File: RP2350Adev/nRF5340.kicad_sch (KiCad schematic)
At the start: 1 part, among them U1 NRF5340-CLAA-R

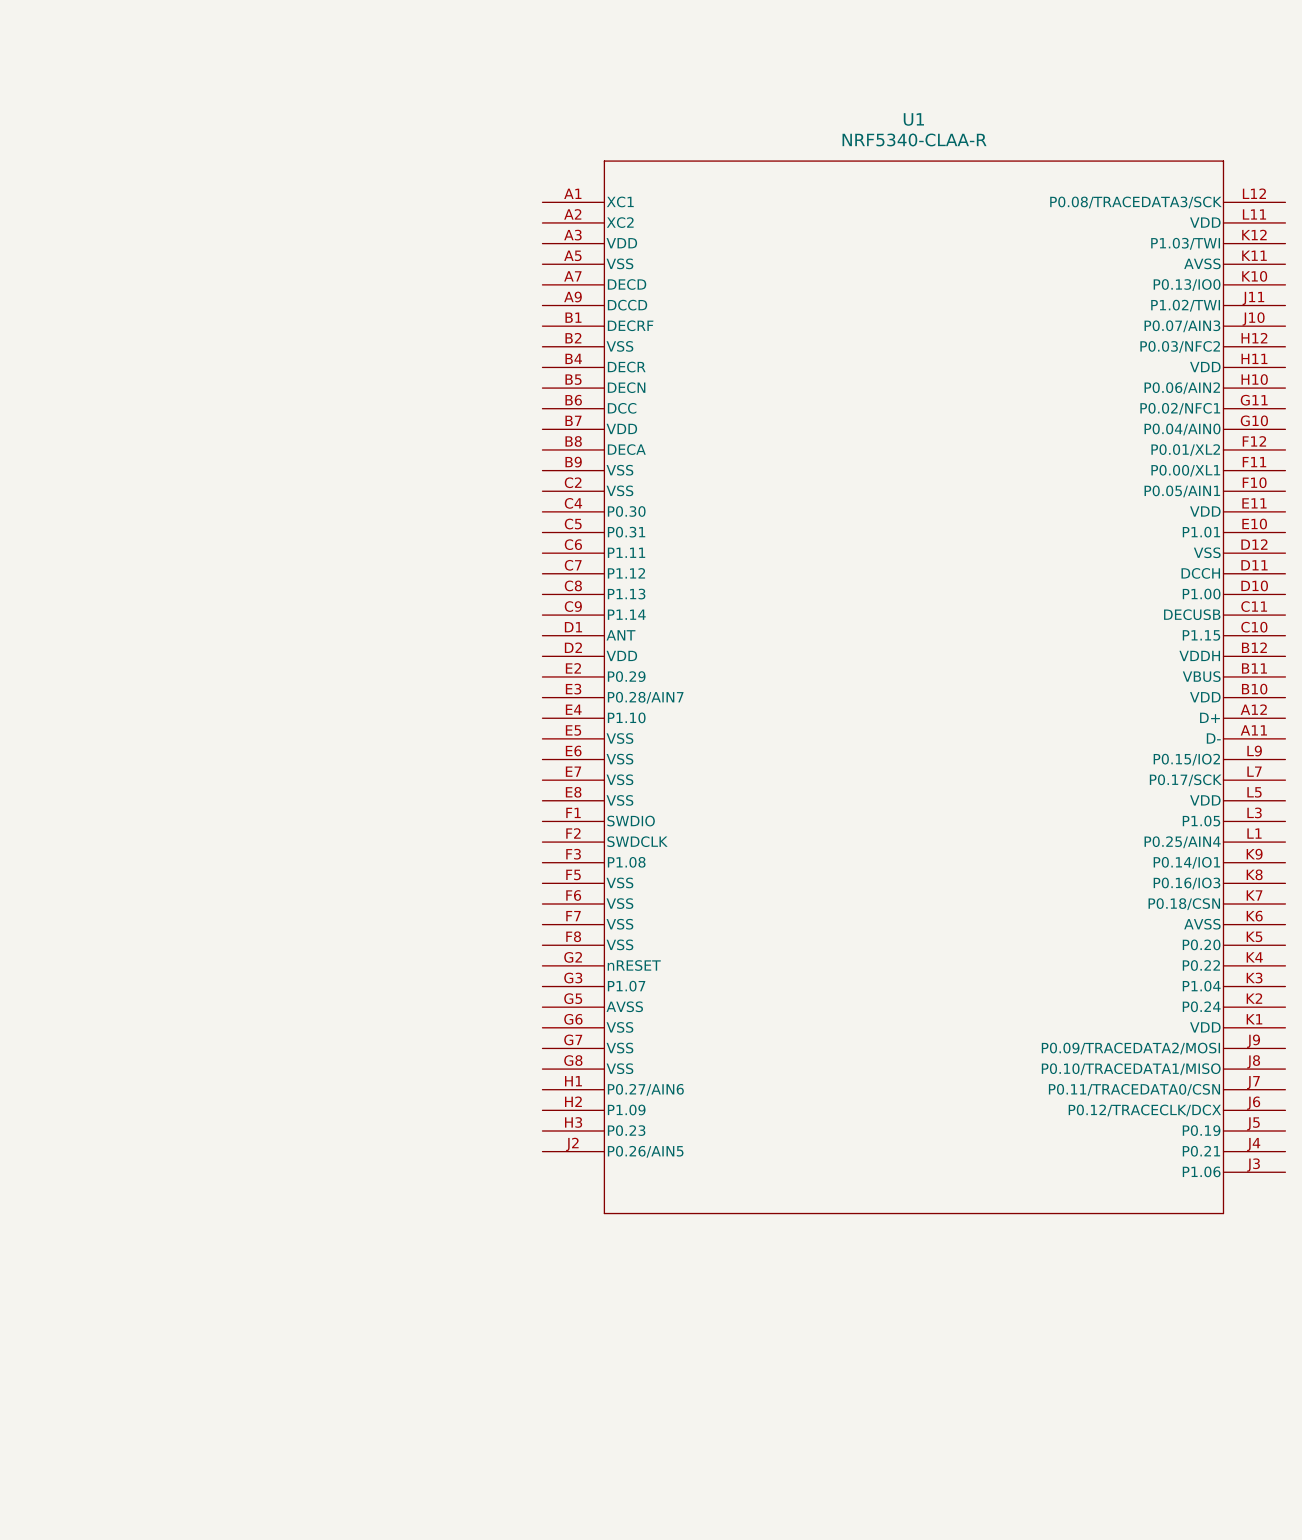
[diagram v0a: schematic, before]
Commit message: Updated nRF5340 work
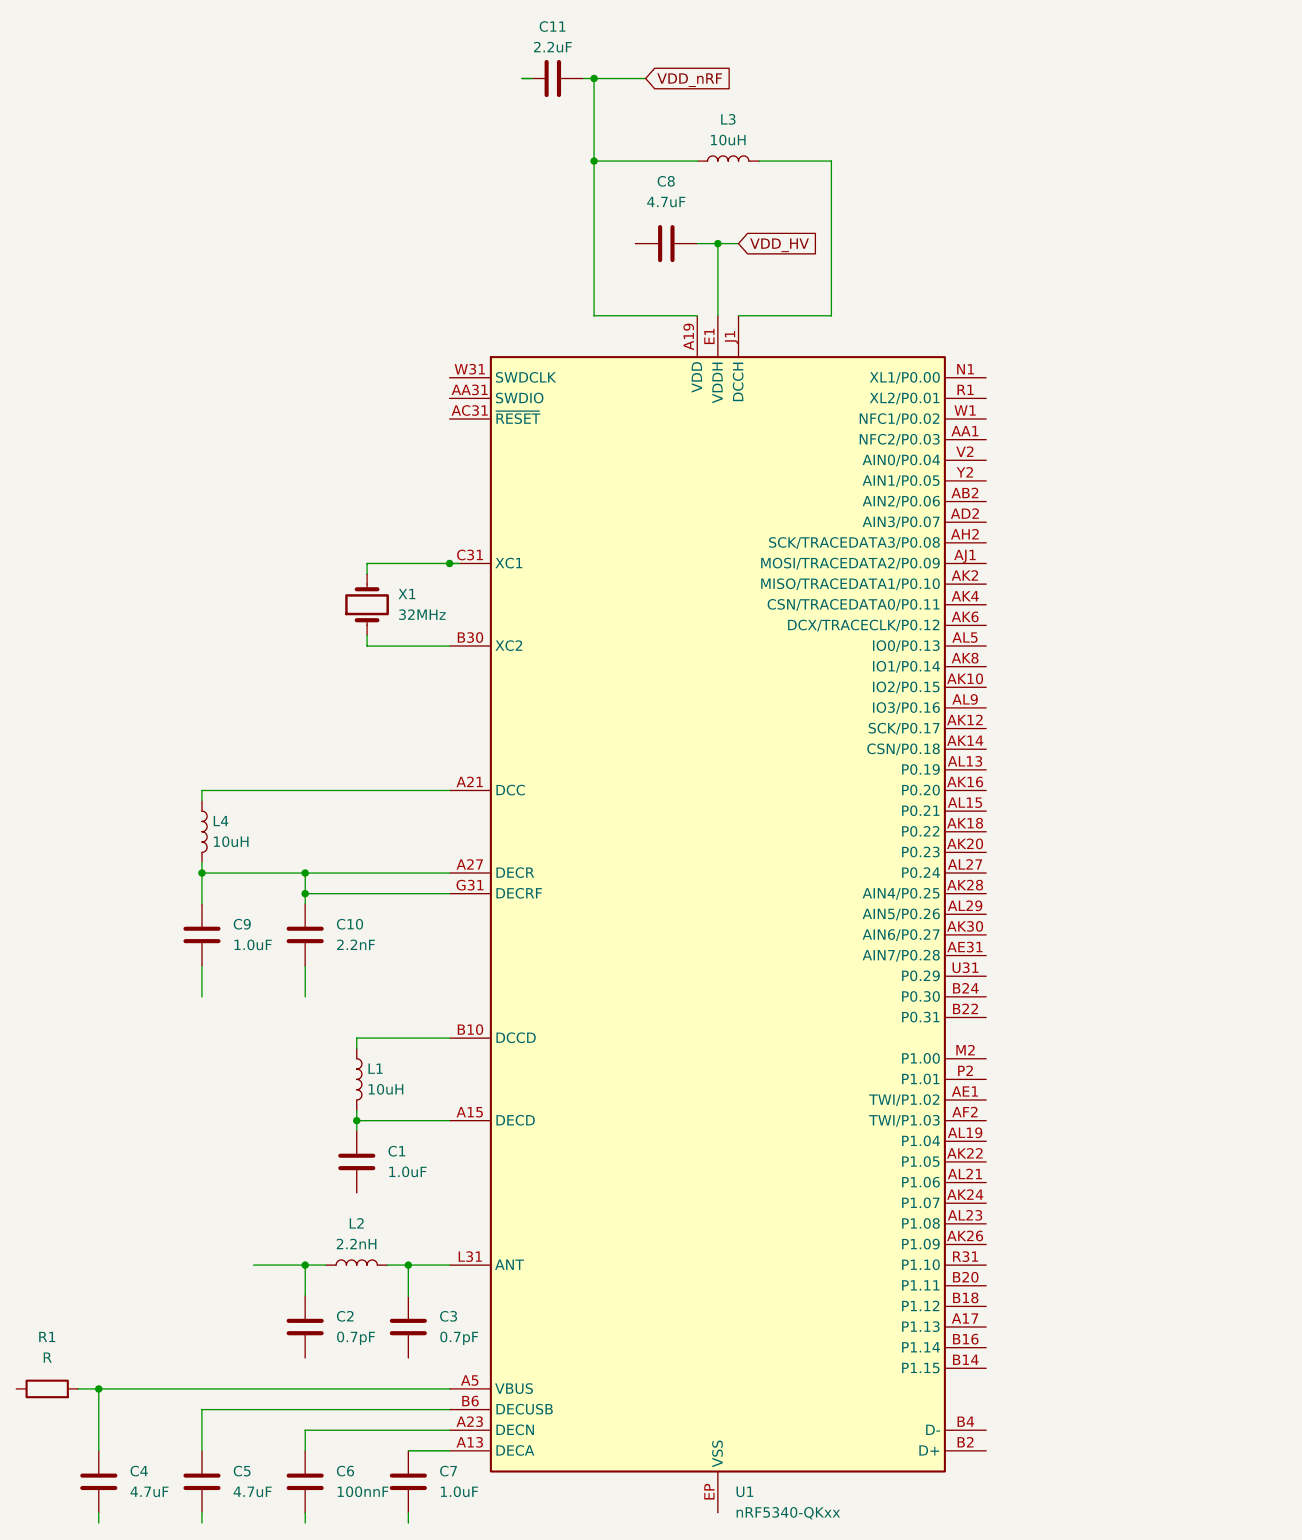
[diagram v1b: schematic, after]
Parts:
- removed U1: NRF5340-CLAA-R, WLCSP95_4.390X3.994_NOR, symbol nRF5340:NRF5340-CLAA-R
- added C1, C7, C9: 1.0uF, symbol Device:C
- added C10: 2.2nF, symbol Device:C
- added C11: 2.2uF, symbol Device:C
- added C2, C3: 0.7pF, symbol Device:C
- added C4, C5, C8: 4.7uF, symbol Device:C
- added C6: 100nnF, symbol Device:C
- added L1, L3, L4: 10uH, symbol Device:L
- added L2: 2.2nH, symbol Device:L
- added R1: R, symbol Device:R
- added U1: nRF5340-QKxx, Package_DFN_QFN:Nordic_AQFN-94-1EP_7x7mm_P0.4mm, symbol MCU_Nordic:nRF5340-QKxx
- added X1: 32MHz, symbol Device:Crystal
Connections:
- new net: C10.1, C9.1, L4.2, U1.A27 (DECR), U1.G31 (DECRF)
- new net: C3.1, L2.2, U1.L31 (ANT)
- new net: C2.1, L2.1
- new net: U1.B30 (XC2), X1.1
- new net: U1.C31 (XC1), X1.2
- new net: C7.1, U1.A13 (DECA)
- new net: C1.1, L1.2, U1.A15 (DECD)
- new net: L4.1, U1.A21 (DCC)
- new net: C6.1, U1.A23 (DECN)
- new net: C4.1, R1.2, U1.A5 (VBUS)
- new net: L1.1, U1.B10 (DCCD)
- new net: C5.1, U1.B6 (DECUSB)
- new net: L3.2, U1.J1 (DCCH)
- new net VDD_HV: C8.2, U1.E1 (VDDH)
- new net VDD_nRF: C11.2, L3.1, U1.A19 (VDD), U1.AC1 (VDD), U1.AG1 (VDD), U1.AJ31 (VDD), U1.AL11 (VDD), U1.AL17 (VDD), U1.AL25 (VDD), U1.AL3 (VDD), U1.AL7 (VDD), U1.B28 (VDD), U1.B8 (VDD), U1.C1 (VDD), U1.E31 (VDD), U1.L1 (VDD), U1.N31 (VDD), U1.U1 (VDD)
